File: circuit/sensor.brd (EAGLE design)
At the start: 12.7 x 25.1 mm, 10 parts, among them IC1 A1302LH

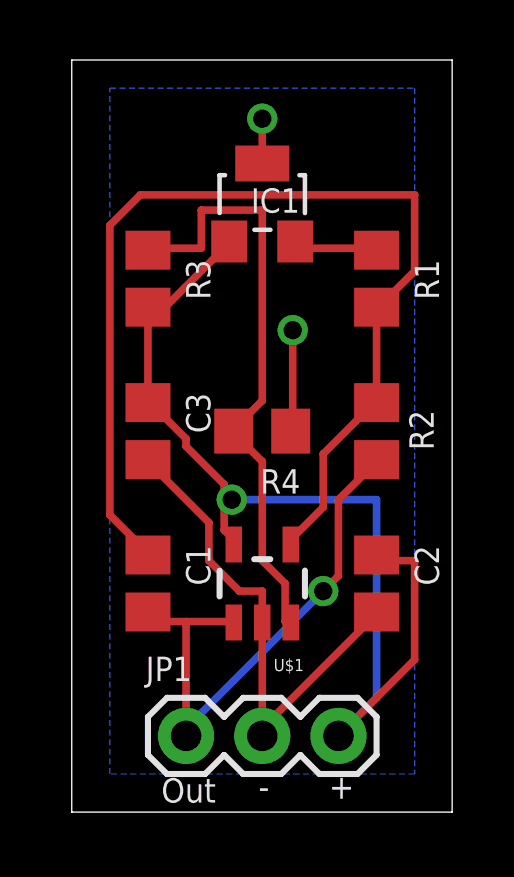
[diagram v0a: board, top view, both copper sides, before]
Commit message: update sensor
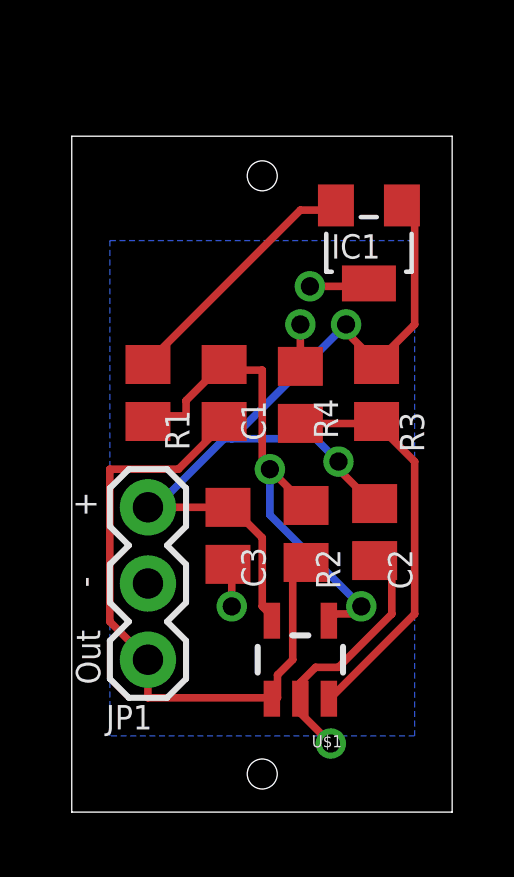
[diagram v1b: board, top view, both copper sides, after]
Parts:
- moved R1 8.52 mm to (2.54, 14.0)
- moved R3 8.52 mm to (10.2, 14.0), turned to 90 degrees
- moved C1 6.84 mm to (5.08, 14.0)
- moved C3 4.39 mm to (5.21, 9.21)
- moved R2 4.16 mm to (7.81, 9.27)
- moved IC1 3.82 mm to (9.91, 18.9), turned to 180 degrees
- moved JP1 2.84 mm to (2.54, 5.08), turned to 90 degrees
- moved U$1 2.84 mm to (7.62, 5.08)
- moved R4 1.75 mm to (7.62, 13.9), turned to 270 degrees
- moved C2 1.72 mm to (10.1, 9.33)
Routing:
- net N$3: track 35.7 -> 17.7 mm, vias 0 -> 2
- net GND: track 21.9 -> 14.0 mm, vias 2 -> 4
- net N$5: track 20.4 -> 13.6 mm
- net N$2: track 2.89 -> 8.70 mm
- net 5V: track 34.8 -> 29.8 mm, vias 1 -> 2
- net N$1: track 18.8 -> 21.9 mm, vias 1 -> 0
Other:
- board size 12.7 x 25.1 mm -> 12.7 x 22.5 mm
